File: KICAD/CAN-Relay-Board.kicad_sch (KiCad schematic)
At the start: 28 parts, among them J1 UPDI Header, J2 Conn_01x04_Female, J3 UART Header, U1 AZ1117-5.0, U2 MCP2551-I-SN, U3 ATtiny414-SS, U5 MCP2515-xSO, Y1 8MHz

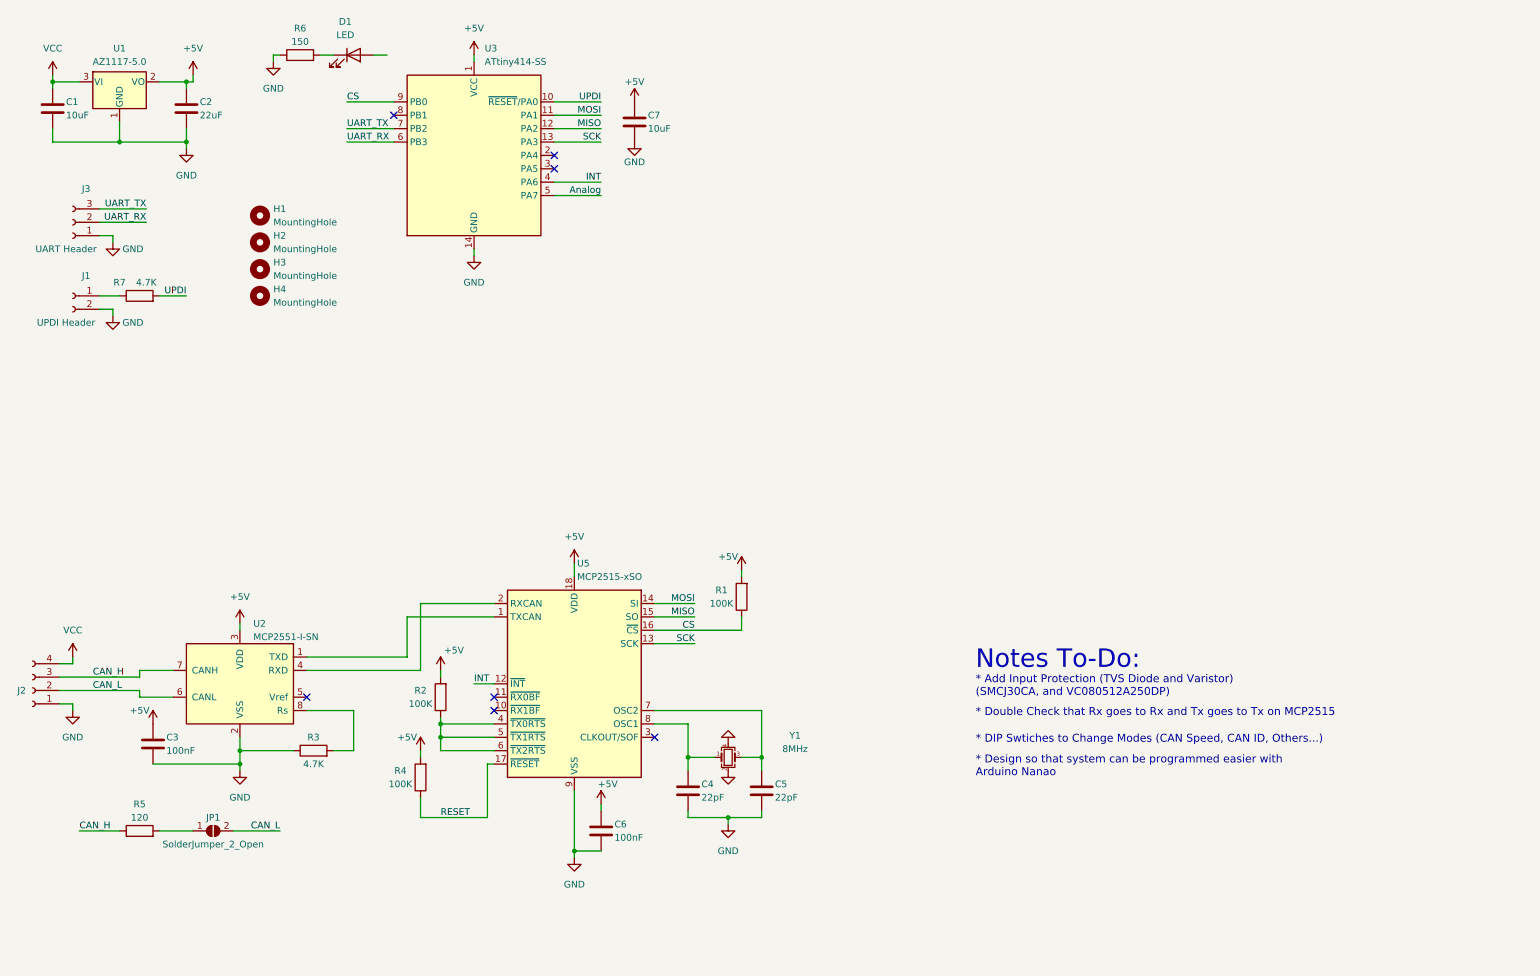
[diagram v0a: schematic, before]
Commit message: Schematic 90% complete
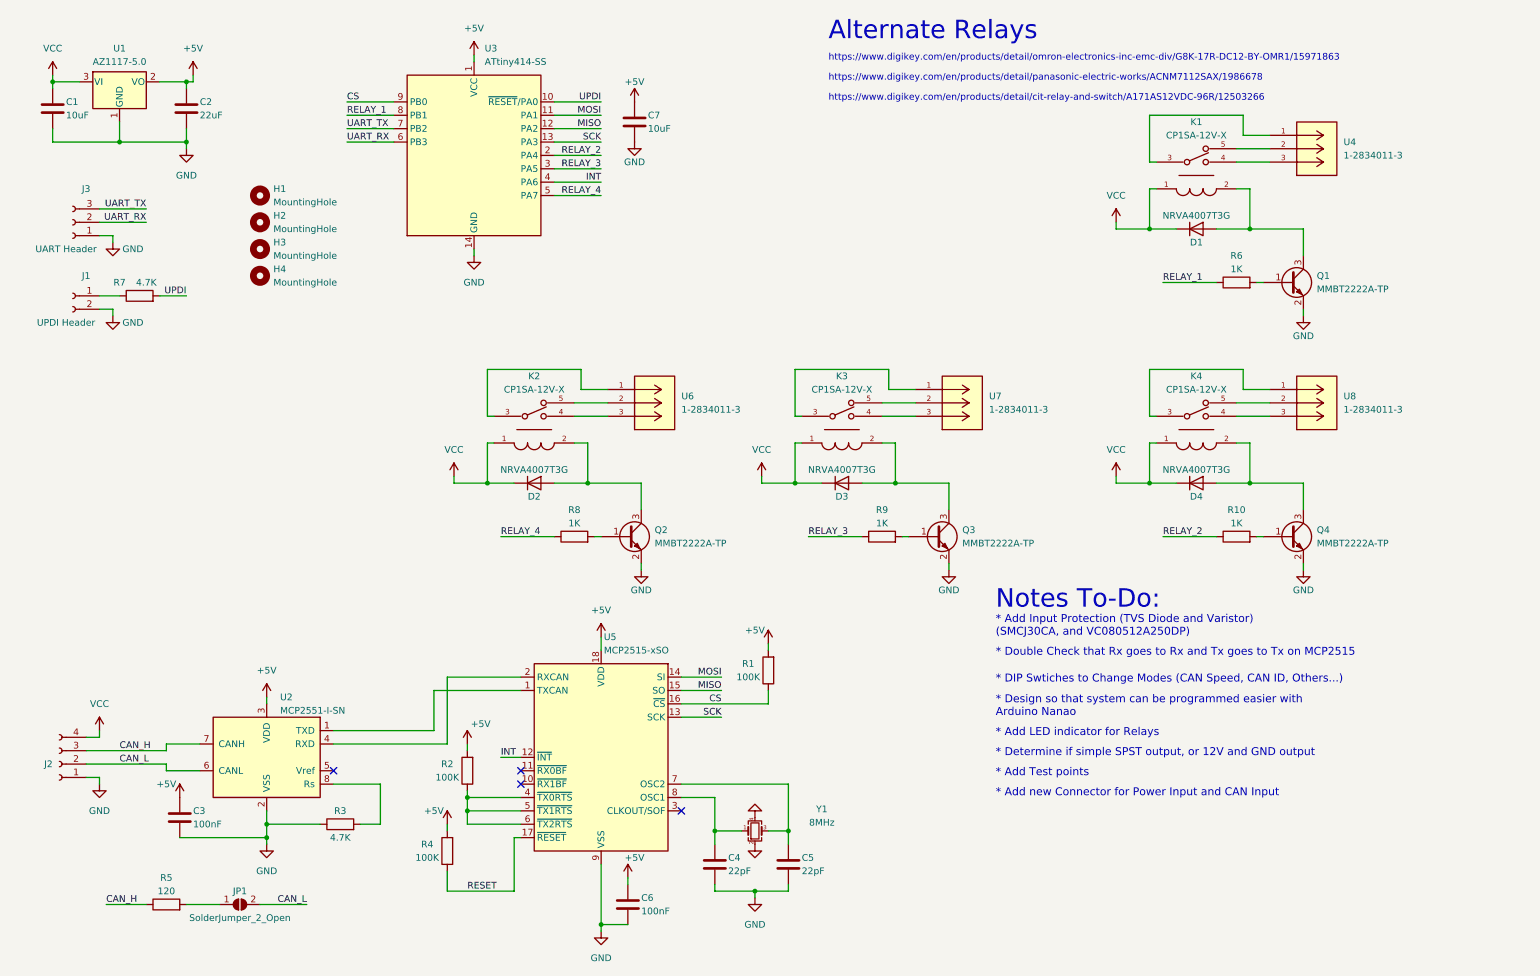
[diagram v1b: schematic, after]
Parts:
- removed D1: LED, LED_SMD:LED_0603_1608Metric_Pad1.05x0.95mm_HandSolder, symbol Device:LED
- added D1, D2, D3, D4: NRVA4007T3G, Diode_SMD:D_SMA, symbol Diode:NRVA4007T3G
- added K1, K2, K3, K4: CP1SA-12V-X, eec:Panasonic-CP1SA-12V-X-MFG, symbol eec:CP1SA-12V-X
- added Q1, Q2, Q3, Q4: MMBT2222A-TP, Package_TO_SOT_SMD:SOT-23, symbol Transistor_BJT:MMBT3904
- added R10, R8, R9: 1K, Resistor_SMD:R_0603_1608Metric_Pad0.98x0.95mm_HandSolder, symbol Device:R
- added U4, U6, U7, U8: 1-2834011-3, 1-2834011-3:CONN_1-2834011-3, symbol 1-2834011-3:1-2834011-3
- R6: value 150 -> 1K; Digi-Key Link https://www.digikey.com/en/products/detail/yageo/RC0603FR-0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 -> (none); Digi-Key PN 311-150HRCT-ND -> (none); Manufacturer PN RC0603FR-07150RL -> (none); Price 0.10 -> (none)
- U2: Digi-Key Link (none) -> https://www.digikey.com/en/products/detail/microchip-techno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; Digi-Key PN (none) -> MCP2551-I/SN-ND; Manufacturer PN (none) -> MCP2551-I/SN; Price (none) -> 1.37
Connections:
- net GND: now also Q1.2 (E), Q2.2 (E), Q3.2 (E), Q4.2 (E); no longer R6.1
- net VCC: now also D1.1 (K), D2.1 (K), D3.1 (K), D4.1 (K), K1.1 (1_COIL), K2.1 (1_COIL), K3.1 (1_COIL), K4.1 (1_COIL)
- net at R6.2: now also Q1.1 (B)
- net RELAY_2: now reaches U3.2 (PA4)
- net RELAY_2: now also R10.1
- net RELAY_3: now reaches U3.3 (PA5)
- net RELAY_3: now also R9.1
- net RELAY_1: now reaches U3.8 (PB1)
- net RELAY_1: now also R6.1
- net Analog renamed RELAY_4
- net RELAY_4: now also R8.1
- new net: Q4.1 (B), R10.2
- new net: D4.2 (A), K4.2 (2_COIL), Q4.3 (C)
- new net: D3.2 (A), K3.2 (2_COIL), Q3.3 (C)
- new net: K4.3 (COM), U8.1
- new net: K4.4 (NO), U8.3
- new net: K4.5 (NC), U8.2
- new net: D1.2 (A), K1.2 (2_COIL), Q1.3 (C)
- new net: K1.3 (COM), U4.1
- new net: K1.4 (NO), U4.3
- new net: K1.5 (NC), U4.2
- new net: K2.3 (COM), U6.1
- new net: K2.5 (NC), U6.2
- new net: K2.4 (NO), U6.3
- new net: D2.2 (A), K2.2 (2_COIL), Q2.3 (C)
- new net: Q2.1 (B), R8.2
- new net: K3.3 (COM), U7.1
- new net: K3.4 (NO), U7.3
- new net: K3.5 (NC), U7.2
- new net: Q3.1 (B), R9.2
- no-connect marks 7 -> 4
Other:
- note added: "* Add LED indicator for Relays"
- note added: "* Add Test points"
- note added: "* Add new Connector for Power Input and CAN Input"
- note added: "* Determine if simple SPST output, or 12V and GND output"
- note added: "Alternate Relays"
- note added: "https://www.digikey.com/en/products/detail/cit-relay-and-switch/A171AS12VDC-96R/12503266"
- note added: "https://www.digikey.com/en/products/detail/omron-electronics-inc-emc-div/G8K-17R-DC12-BY-OMR1/15971863"
- note added: "https://www.digikey.com/en/products/detail/panasonic-electric-works/ACNM7112SAX/1986678"
- moved on the sheet: C3, C4, C5, C6, H1, H2, H3, H4, J2, JP1, R1, R2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
